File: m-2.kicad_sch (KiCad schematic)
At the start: 19 parts, among them J503 Bus_M.2_1-2199230-6, M503 Mech_M2_2280_H2.5mm

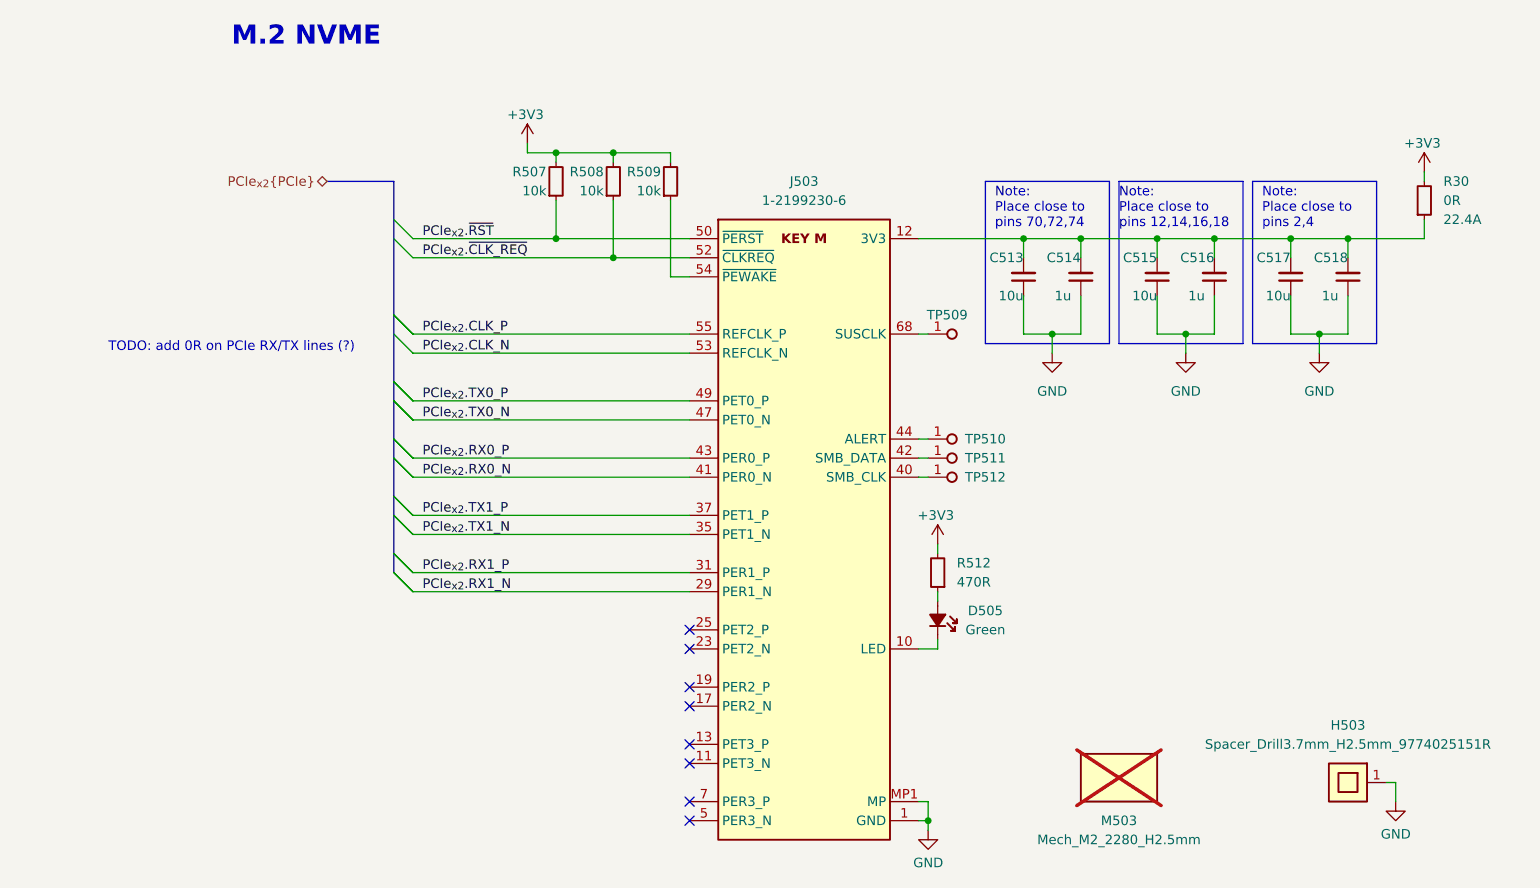
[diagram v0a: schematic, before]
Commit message: [#100765] Update schematic
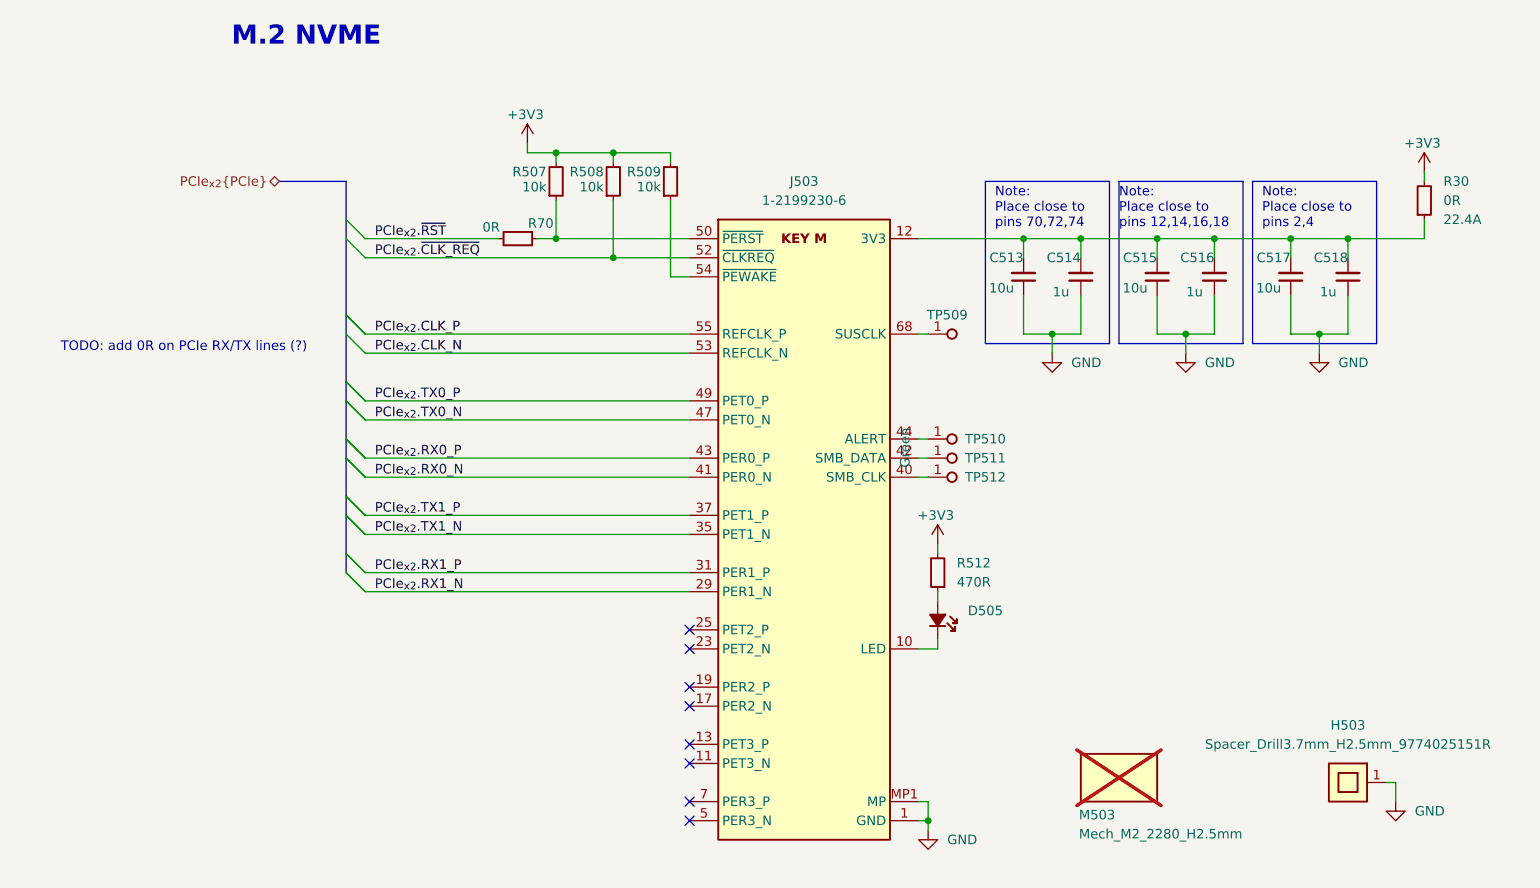
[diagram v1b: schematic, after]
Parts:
- added R70: R_0R_0402, antmicro-footprints:R_0402_1005Metric, symbol antmicroResistors0402:R_0R_0402
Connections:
- net PCIe_{x2}.~{RST}: now also R70.2; no longer J503.50 (~{PERST}), R507.1
- new net: J503.50 (~{PERST}), R507.1, R70.1
